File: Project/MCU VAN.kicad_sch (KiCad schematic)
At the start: 10 parts, among them U59 STM32F072CBT6

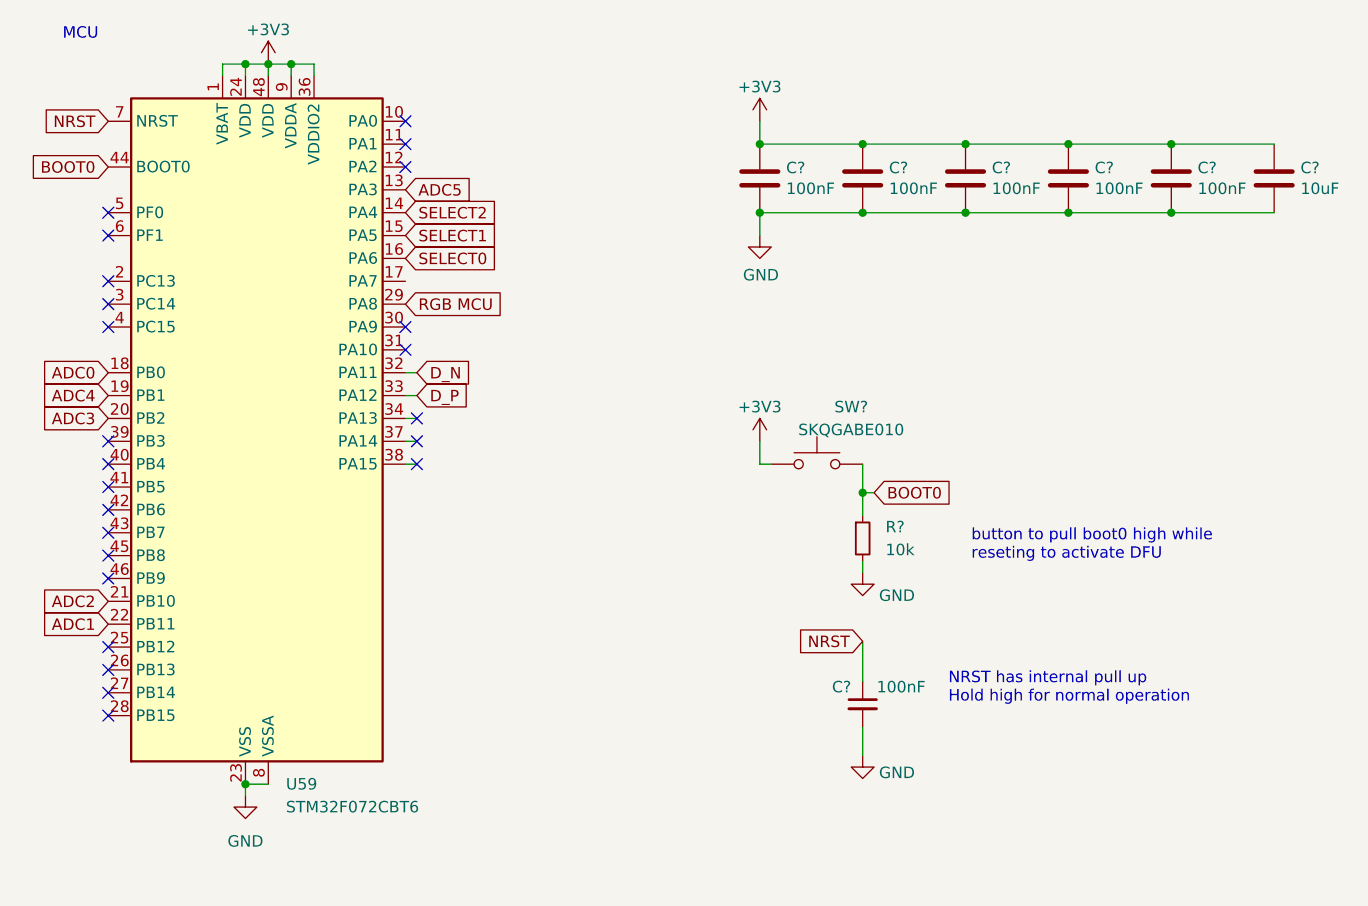
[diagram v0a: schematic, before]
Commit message: pin revision
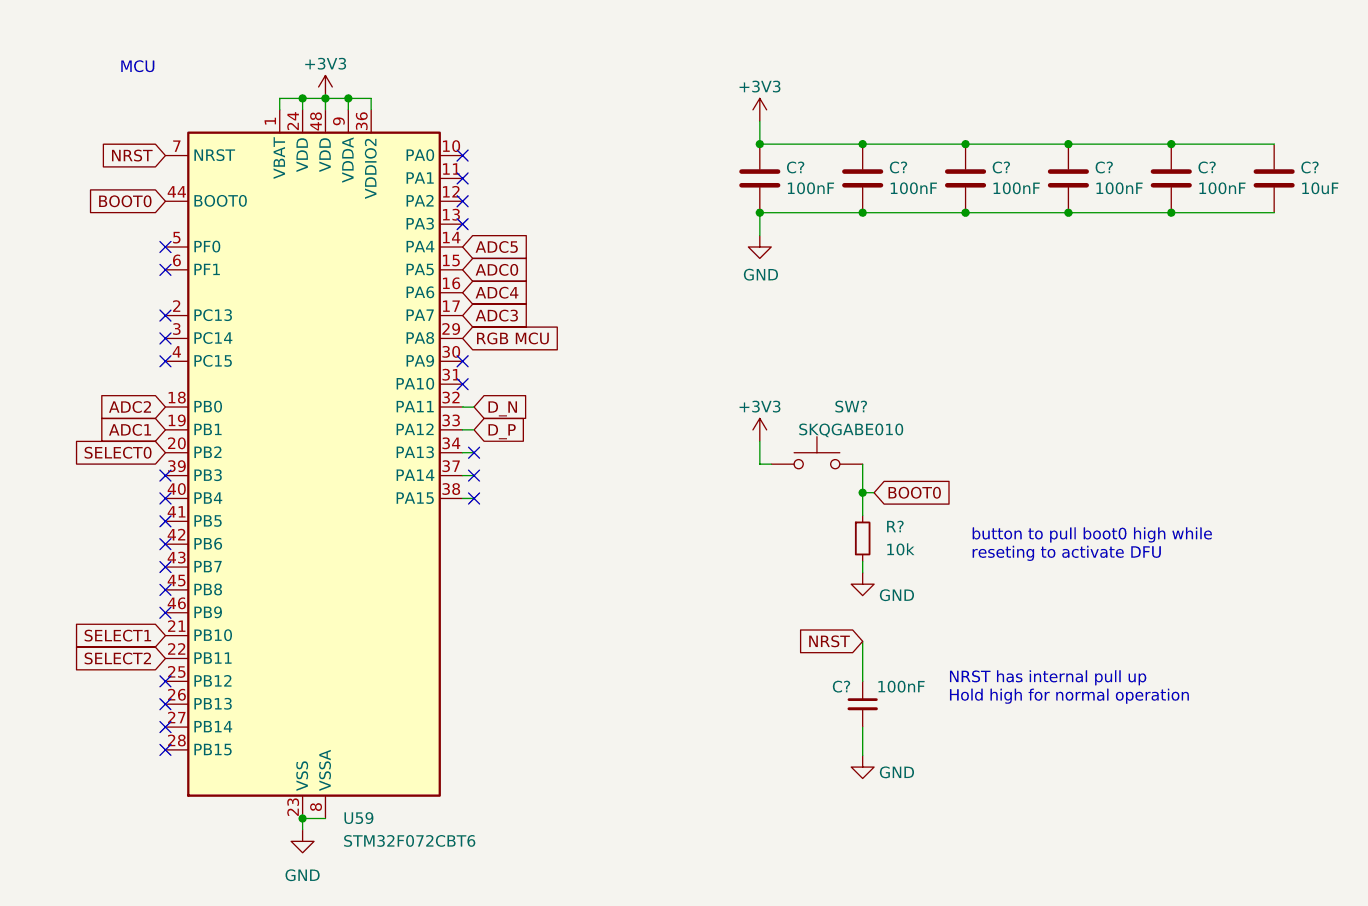
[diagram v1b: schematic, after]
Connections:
- net ADC0: now also U59.15 (PA5); no longer U59.18 (PB0)
- net ADC1: now also U59.19 (PB1); no longer U59.22 (PB11)
- net ADC2: now also U59.18 (PB0); no longer U59.21 (PB10)
- net ADC3: now also U59.17 (PA7); no longer U59.20 (PB2)
- net ADC4: now also U59.16 (PA6); no longer U59.19 (PB1)
- net ADC5: now also U59.14 (PA4); no longer U59.13 (PA3)
- net SELECT0: now also U59.20 (PB2); no longer U59.16 (PA6)
- net SELECT1: now also U59.21 (PB10); no longer U59.15 (PA5)
- net SELECT2: now also U59.22 (PB11); no longer U59.14 (PA4)
- no-connect marks 24 -> 25
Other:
- moved on the sheet: U59
